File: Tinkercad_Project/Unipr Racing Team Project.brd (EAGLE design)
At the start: 128.2 x 112.8 mm, 3 parts, among them U1 ARDUINO-UNO-R3-SHIELD

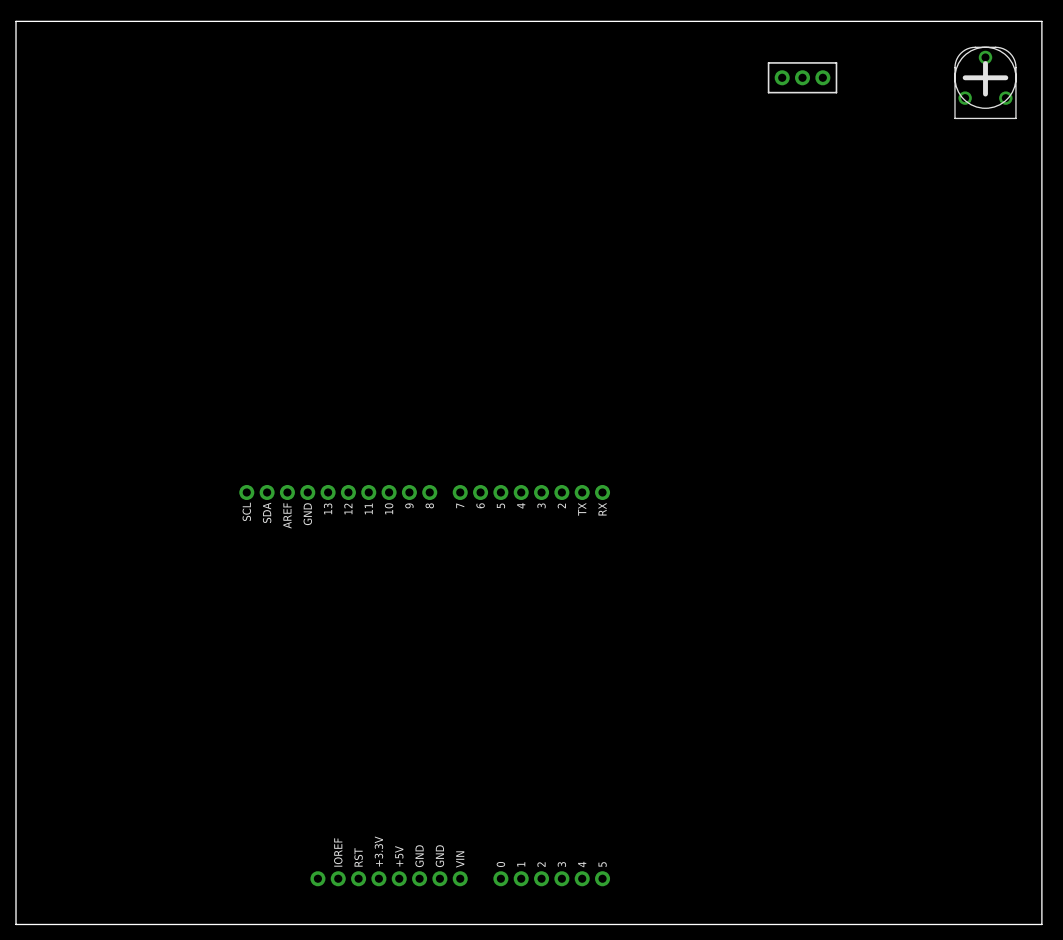
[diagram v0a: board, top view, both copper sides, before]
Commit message: finaly
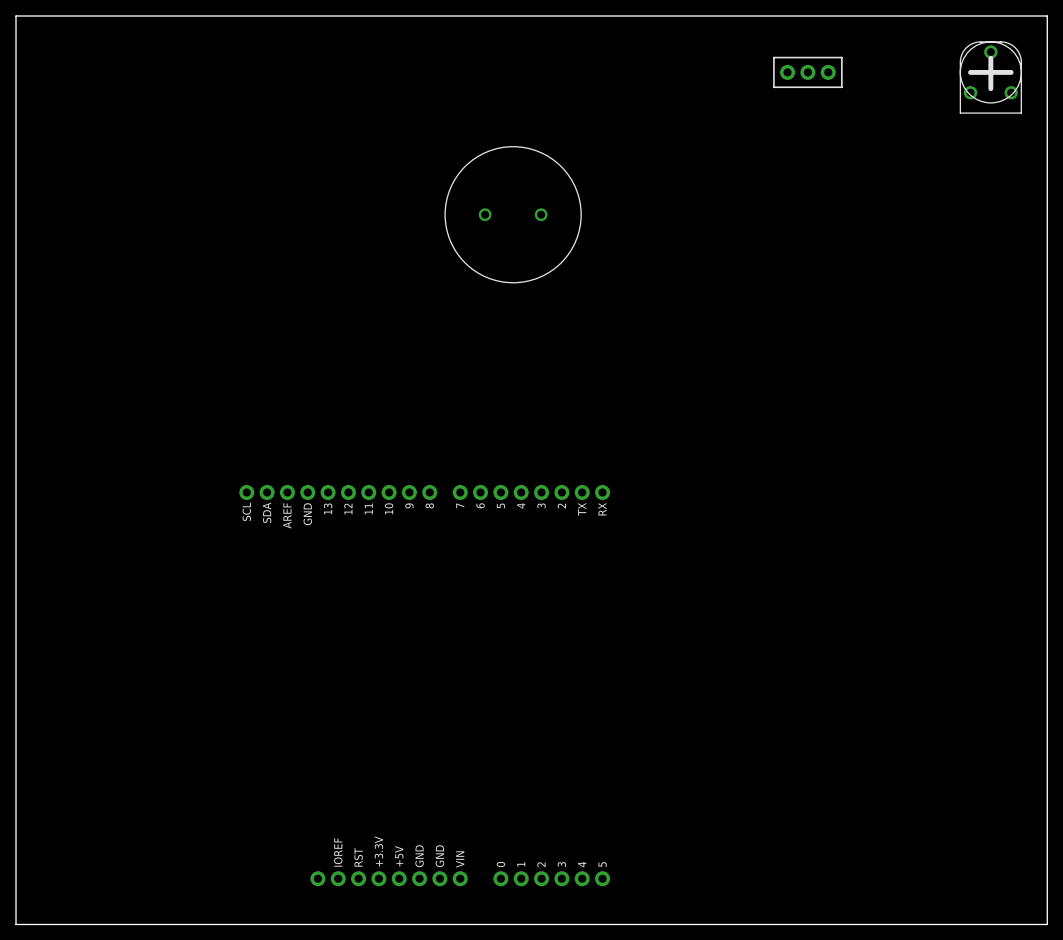
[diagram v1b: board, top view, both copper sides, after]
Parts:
- added PIEZO1: PIEZO, Tinkercad:PIEZO
- moved RPOT1 0.95 mm to (121.8, 106.5)
- moved S1 0.95 mm to (98.9, 106.5)
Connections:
- new net U1_D9: PIEZO1.1, U1.D9
- net U1_GND: now also PIEZO1.2
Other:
- board size 128.2 x 112.8 mm -> 128.9 x 113.5 mm
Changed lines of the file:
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@@
 <board>
 <plain>
-<wire x1="0" y1="0" x2="128.1814845500015" y2="0" width="0" layer="20"/>
-<wire x1="128.1814845500015" y1="0" x2="128.1814845500015" y2="112.83930567513217" width="0" layer="20"/>
-<wire x1="128.1814845500015" y1="112.83930567513217" x2="0" y2="112.83930567513217" width="0" layer="20"/>
-<wire x1="0" y1="112.83930567513217" x2="0" y2="0" width="0" layer="20"/>
+<wire x1="0" y1="0" x2="128.85228875274993" y2="0" width="0" layer="20"/>
+<wire x1="128.85228875274993" y1="0" x2="128.85228875274993" y2="113.51010987788058" width="0" layer="20"/>
+<wire x1="128.85228875274993" y1="113.51010987788058" x2="0" y2="113.51010987788058" width="0" layer="20"/>
+<wire x1="0" y1="113.51010987788058" x2="0" y2="0" width="0" layer="20"/>
 </plain>
 <attributes/>
@@
 </autorouter>
 <elements>
-<element name="RPOT1" library="Tinkercad" package="HA-06-SM065" package3d_urn="urn:adsk.eagle:package:31496083/2" value="5k" x="121.133" y="105.7908" smashed="yes"/>
+<element name="S1" library="Tinkercad" package="SWITCH-SPDT-PTH-8.5X3.7MM" package3d_urn="urn:adsk.eagle:package:32246661/2" value="TOGGLE" x="98.9438" y="106.4616" smashed="yes"/>
+<element name="RPOT1" library="Tinkercad" package="HA-06-SM065" package3d_urn="urn:adsk.eagle:package:31496083/2" value="5k" x="121.8038" y="106.4616" smashed="yes"/>
 <element name="U1" library="Tinkercad" package="ARDUINO-UNO-R3-SHIELD" package3d_urn="urn:adsk.eagle:package:32092383/4" value="ARDUINO-UNO-R3-SHIELD" x="47.885" y="29.845" rot="R270" smashed="yes"/>
-<element name="S1" library="Tinkercad" package="SWITCH-SPDT-PTH-8.5X3.7MM" package3d_urn="urn:adsk.eagle:package:32246661/2" value="TOGGLE" x="98.273" y="105.7908" smashed="yes"/>
+<element name="PIEZO1" library="Tinkercad" package="PIEZO" package3d_urn="urn:adsk.eagle:package:32623992/2" value="PIEZO" x="62.1138" y="88.6816" smashed="yes"/>
 </elements>
 <signals>
@@
 <contactref element="RPOT1" pad="3"/>
 <contactref element="S1" pad="3"/>
+<contactref element="PIEZO1" pad="2"/>
 <wire x1="50.425" y1="5.715" x2="52.965" y2="5.715" width="0" layer="19" extent="1-1"/>
 <wire x1="50.425" y1="5.715" x2="36.455" y2="53.975" width="0" layer="19" extent="1-1"/>
-<wire x1="36.455" y1="53.975" x2="100.813" y2="105.7908" width="0" layer="19" extent="1-1"/>
-<wire x1="123.673" y1="103.2508" x2="100.813" y2="105.7908" width="0" layer="19" extent="1-1"/>
+<wire x1="36.455" y1="53.975" x2="65.6138" y2="88.6816" width="0" layer="19" extent="1-1"/>
+<wire x1="101.4838" y1="106.4616" x2="65.6138" y2="88.6816" width="0" layer="19" extent="1-1"/>
+<wire x1="124.3438" y1="103.9216" x2="101.4838" y2="106.4616" width="0" layer="19" extent="1-1"/>
 </signal>
 <signal name="U1_A1">
@@
 <contactref element="U1" pad="A1"/>
 <contactref element="RPOT1" pad="1"/>
-<wire x1="98.273" y1="105.7908" x2="118.593" y2="103.2508" width="0" layer="19" extent="1-1"/>
-<wire x1="98.273" y1="105.7908" x2="63.125" y2="5.715" width="0" layer="19" extent="1-1"/>
+<wire x1="98.9438" y1="106.4616" x2="119.2638" y2="103.9216" width="0" layer="19" extent="1-1"/>
+<wire x1="98.9438" y1="106.4616" x2="63.125" y2="5.715" width="0" layer="19" extent="1-1"/>
+</signal>
+<signal name="U1_5V">
+<contactref element="U1" pad="5V"/>
+<contactref element="S1" pad="1"/>
+<wire x1="47.885" y1="5.715" x2="96.4038" y2="106.4616" width="0" layer="19" extent="1-1"/>
 </signal>
 <signal name="U1_A0">
 <contactref element="U1" pad="A0"/>
 <contactref element="RPOT1" pad="2"/>
-<wire x1="60.585" y1="5.715" x2="121.133" y2="108.3308" width="0" layer="19" extent="1-1"/>
-</signal>
-<signal name="U1_5V">
-<contactref element="U1" pad="5V"/>
-<contactref element="S1" pad="1"/>
-<wire x1="47.885" y1="5.715" x2="95.733" y2="105.7908" width="0" layer="19" extent="1-1"/>
+<wire x1="60.585" y1="5.715" x2="121.8038" y2="109.0016" width="0" layer="19" extent="1-1"/>
+</signal>
+<signal name="U1_D9">
+<contactref element="PIEZO1" pad="1"/>
+<contactref element="U1" pad="D9"/>
+<wire x1="58.6138" y1="88.6816" x2="49.155" y2="53.975" width="0" layer="19" extent="1-1"/>
 </signal>
 </signals>
